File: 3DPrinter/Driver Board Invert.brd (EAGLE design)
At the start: 127.6 x 42.2 mm, 21 parts, among them X1 CON-7.62-02P, X2 CON-XH-04

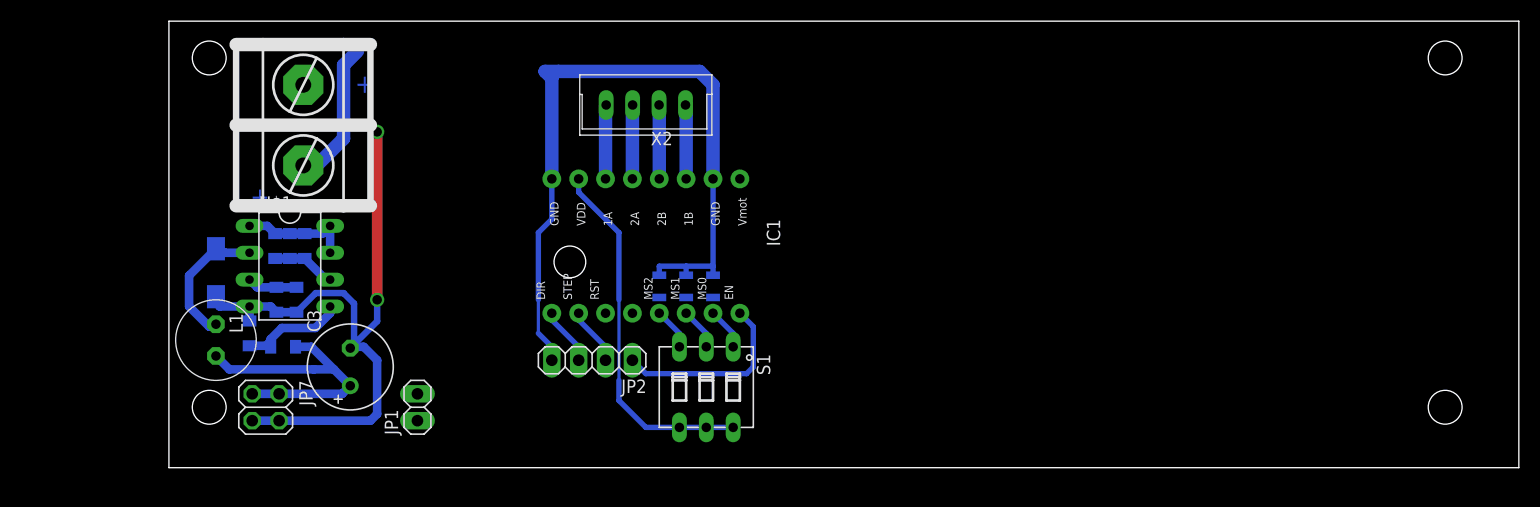
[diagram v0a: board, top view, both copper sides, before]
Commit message: _
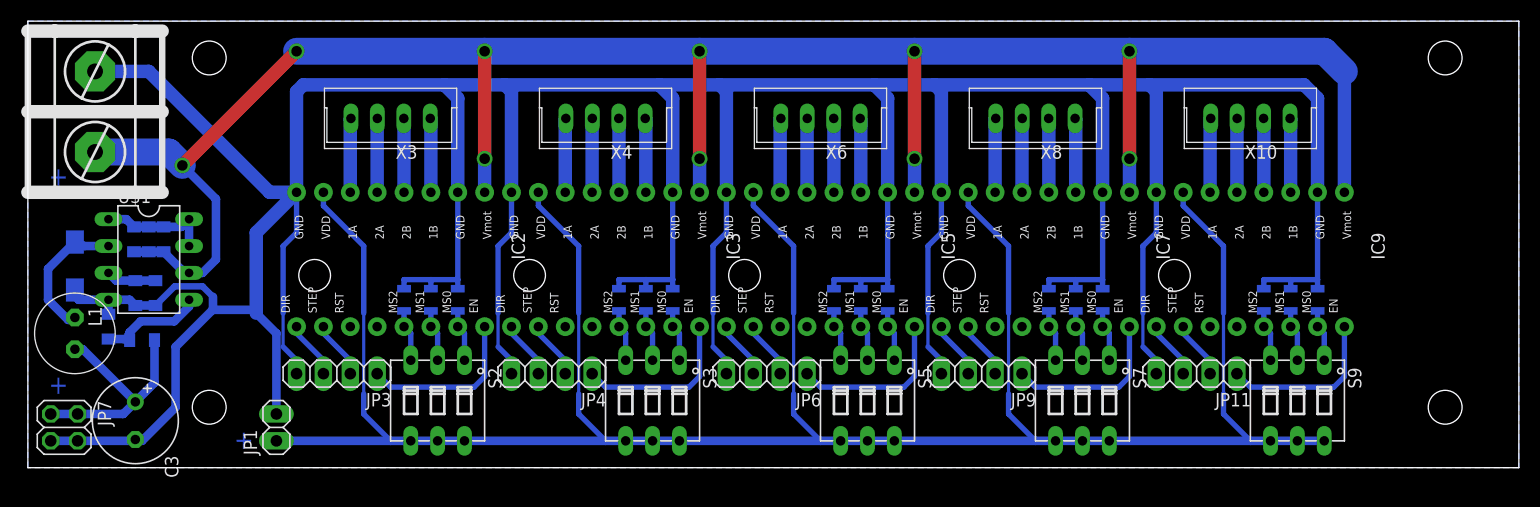
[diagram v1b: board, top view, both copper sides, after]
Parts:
- removed IC1: (no value), Flamberm:DRV-ST820-REV
- removed JP2: (no value), pinhead:1X04
- removed R1, R2, R3: 15K, Flamberm:RESC2012X50
- removed S1: (no value), Namenlos:DIP03YL
- removed X2: CON-XH-04, Namenlos:XH-04
- added IC2, IC3, IC5, IC7, IC9: (no value), Flamberm:DRV-ST820-REV
- added JP11, JP3, JP4, JP6, JP9: (no value), pinhead:1X04
- added R13, R14, R15, R24, R25, R26, R30, R31, R32, R4, R5, R6, R7, R8, R9: 15K, Flamberm:RESC2012X50
- added S2, S3, S5, S7, S9: (no value), Namenlos:DIP03YL
- added X10, X3, X4, X6, X8: CON-XH-04, Namenlos:XH-04
- moved C3 20.9 mm to (-3.17, 41.9), turned to 270 degrees
- moved X1 19.7 mm to (-6.99, 71.1)
- moved JP7 19.1 mm to (-9.91, 41.3)
- moved JP1 13.5 mm to (10.2, 41.3)
- moved C1 13.4 mm to (-3.17, 54.0)
- moved D1 13.4 mm to (-8.89, 56.5)
- moved L1 13.4 mm to (-8.89, 50.2)
- moved R16 13.4 mm to (-0.51, 59.1)
- moved R19 13.4 mm to (-5.71, 50.8)
- moved R20 13.4 mm to (-2.54, 49.5)
- moved C2 13.4 mm to (-1.27, 54.0)
- moved R17 13.4 mm to (-1.91, 59.1)
- moved R18 13.4 mm to (-3.30, 59.1)
- moved U$1 13.4 mm to (-1.91, 57.1)
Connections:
- removed net N$1: IC1.EN, JP2.1
- removed net N$12: IC1.2A, X2.3
- removed net N$13: IC1.1A, X2.4
- removed net N$2: IC1.STEP, JP2.2
- removed net N$3: IC1.DIR, JP2.3
- removed net N$4: IC1.1B, X2.1
- removed net N$5: IC1.MS0, R3.2, S1.1
- removed net N$6: IC1.MS1, R2.2, S1.2
- removed net N$7: IC1.MS2, R1.2, S1.3
- removed net N$8: IC1.2B, X2.2
- new net N$10: IC2.STEP, JP3.2
- new net N$11: IC2.DIR, JP3.3
- new net N$14: IC2.1B, X3.1
- new net N$15: IC2.2B, X3.2
- new net N$16: IC2.2A, X3.3
- new net N$17: IC2.1A, X3.4
- new net N$18: IC2.MS0, R6.2, S2.1
- new net N$19: IC2.MS1, R5.2, S2.2
- new net N$20: IC2.MS2, R4.2, S2.3
- new net N$21: IC3.EN, JP4.1
- new net N$22: IC3.STEP, JP4.2
- new net N$23: IC3.DIR, JP4.3
- new net N$24: IC3.1B, X4.1
- new net N$25: IC3.2B, X4.2
- new net N$26: IC3.2A, X4.3
- new net N$27: IC3.1A, X4.4
- new net N$28: IC3.MS0, R9.2, S3.1
- new net N$29: IC3.MS1, R8.2, S3.2
- new net N$30: IC3.MS2, R7.2, S3.3
- new net N$41: IC5.EN, JP6.1
- new net N$42: IC5.STEP, JP6.2
- new net N$43: IC5.DIR, JP6.3
- new net N$44: IC5.1B, X6.1
- new net N$45: IC5.2B, X6.2
- new net N$46: IC5.2A, X6.3
- new net N$47: IC5.1A, X6.4
- new net N$48: IC5.MS0, R15.2, S5.1
- new net N$49: IC5.MS1, R14.2, S5.2
- new net N$50: IC5.MS2, R13.2, S5.3
- new net N$65: IC7.EN, JP9.1
- new net N$66: IC7.STEP, JP9.2
- new net N$67: IC7.DIR, JP9.3
- new net N$68: IC7.1B, X8.1
- new net N$69: IC7.2B, X8.2
- new net N$70: IC7.2A, X8.3
- new net N$71: IC7.1A, X8.4
- new net N$72: IC7.MS0, R26.2, S7.1
- new net N$73: IC7.MS1, R25.2, S7.2
- new net N$74: IC7.MS2, R24.2, S7.3
- new net N$85: IC9.EN, JP11.1
- new net N$86: IC9.STEP, JP11.2
- new net N$87: IC9.DIR, JP11.3
- new net N$88: IC9.1B, X10.1
- new net N$89: IC9.2B, X10.2
- new net N$9: IC2.EN, JP3.1
- new net N$90: IC9.2A, X10.3
- new net N$91: IC9.1A, X10.4
- new net N$92: IC9.MS0, R32.2, S9.1
- new net N$93: IC9.MS1, R31.2, S9.2
- new net N$94: IC9.MS2, R30.2, S9.3
- net +24V: now also IC2.VM, IC3.VM, IC5.VM, IC7.VM, IC9.VM; no longer IC1.VM
- net +3V3: now also IC2.VDD, IC3.VDD, IC5.VDD, IC7.VDD, IC9.VDD, S2.4, S2.5, S2.6, S3.4, S3.5, S3.6, S5.4, S5.5, S5.6, S7.4, S7.5, S7.6, S9.4, S9.5, S9.6; no longer IC1.VDD, S1.4, S1.5, S1.6
- net GND: now also IC2.GND@1, IC2.GND@2, IC3.GND@1, IC3.GND@2, IC5.GND@1, IC5.GND@2, IC7.GND@1, IC7.GND@2, IC9.GND@1, IC9.GND@2, JP11.4, JP3.4, JP4.4, JP6.4, JP9.4, R13.1, R14.1, R15.1, R24.1, R25.1, R26.1, R30.1, R31.1, R32.1, R4.1, R5.1, R6.1, R7.1, R8.1, R9.1; no longer IC1.GND@1, IC1.GND@2, JP2.4, R1.1, R2.1, R3.1
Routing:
- net GND: track 132.5 -> 464.3 mm, vias 2 -> 0
- net +3V3: track 34.4 -> 229.7 mm
- net +24V: track 19.7 -> 208.0 mm, vias 0 -> 10
- net N$1: track 17.8 -> 0.00 mm
- net N$65: track 0.00 -> 15.8 mm
- net N$9: track 0.00 -> 15.8 mm
- net N$85: track 0.00 -> 15.8 mm
- net N$41: track 0.00 -> 15.8 mm
- net N$21: track 0.00 -> 15.8 mm
- net N$91: track 0.00 -> 7.01 mm
- net N$88: track 0.00 -> 7.01 mm
- net N$71: track 0.00 -> 7.01 mm
- net N$47: track 0.00 -> 7.01 mm
- net N$44: track 0.00 -> 7.01 mm
- net N$4: track 7.01 -> 0.00 mm
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- added copper zone on layer 16, net GND
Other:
- board size 127.6 x 42.2 mm -> 140.9 x 42.2 mm
